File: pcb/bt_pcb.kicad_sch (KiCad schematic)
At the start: 1 part, among them IC4 STM32H750VBT6

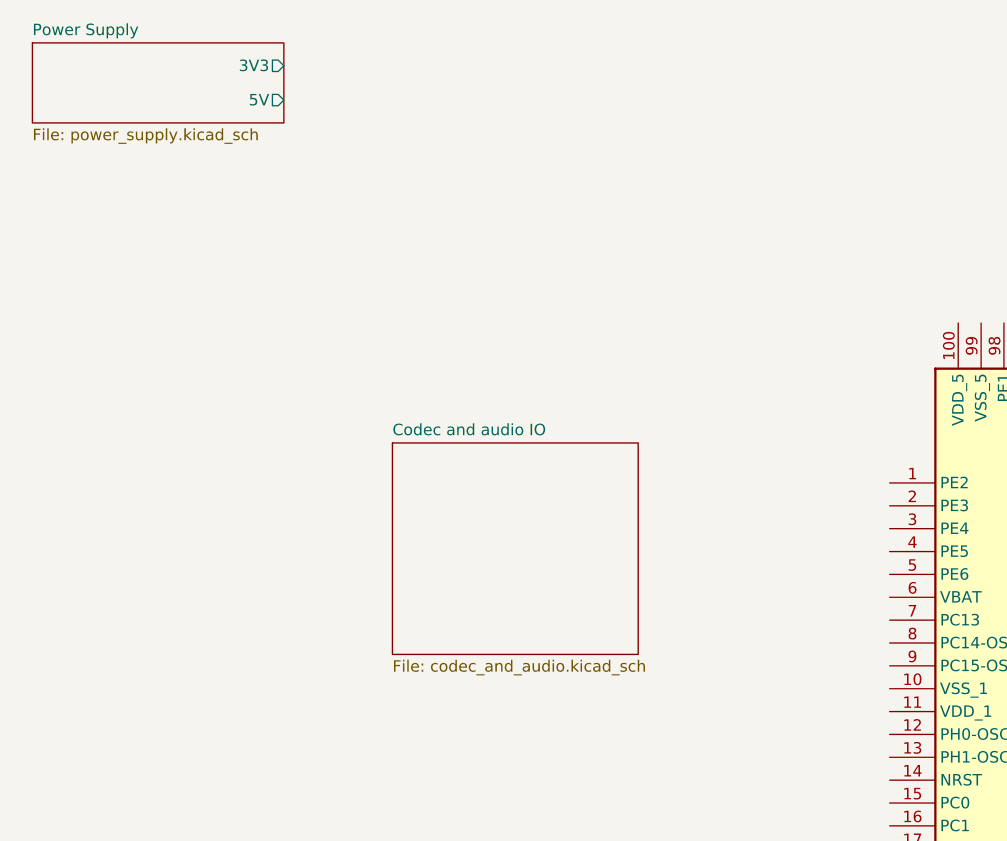
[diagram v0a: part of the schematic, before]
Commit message: progress on audio pcb
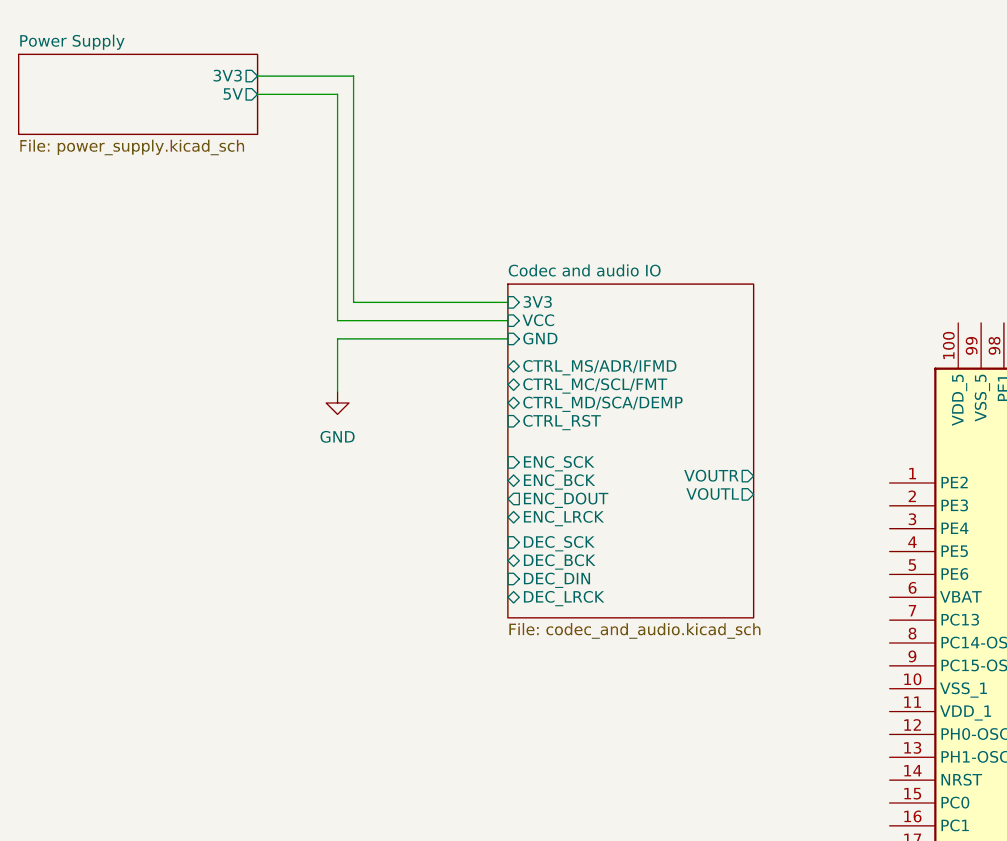
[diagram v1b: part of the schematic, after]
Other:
- sheet Codec and audio IO ports: added 3V3, CTRL_MC/SCL/FMT, CTRL_MD/SCA/DEMP, CTRL_MS/ADR/IFMD, CTRL_RST, DEC_BCK, DEC_DIN, DEC_LRCK, DEC_SCK, ENC_BCK, ENC_DOUT, ENC_LRCK, ENC_SCK, GND, VCC, VOUTL, VOUTR; removed none
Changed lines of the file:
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@@
 (kicad_sch (version 20230121) (generator eeschema)
   (paper "A4")
+  (wire (pts (xy 71.882 67.564) (xy 89.027 67.564))
+    (stroke (width 0) (type default))
+  )
+  (wire (pts (xy 61.214 42.418) (xy 71.882 42.418))
+    (stroke (width 0) (type default))
+  )
+  (wire (pts (xy 71.882 42.418) (xy 71.882 67.564))
+    (stroke (width 0) (type default))
+  )
+  (wire (pts (xy 89.027 69.596) (xy 70.104 69.596))
+    (stroke (width 0) (type default))
+  )
+  (wire (pts (xy 70.104 71.628) (xy 70.104 77.47))
+    (stroke (width 0) (type default))
+  )
+  (wire (pts (xy 70.104 69.596) (xy 70.104 44.45))
+    (stroke (width 0) (type default))
+  )
+  (wire (pts (xy 61.214 44.45) (xy 70.104 44.45))
+    (stroke (width 0) (type default))
+  )
+  (wire (pts (xy 89.027 71.628) (xy 70.104 71.628))
+    (stroke (width 0) (type default))
+  )
+  (symbol (lib_id "power:GND") (at 70.104 77.47 0) (unit 1)
+    (in_bom yes) (on_board yes) (dnp no) (fields_autoplaced)
+    (property "Reference" "#PWR07" (at 70.104 83.82 0)
+      (effects (font (size 1.27 1.27)) hide)
+    )
+    (property "Value" "GND" (at 70.104 82.55 0)
+      (effects (font (size 1.27 1.27)))
+    )
+    (property "Footprint" "" (at 70.104 77.47 0)
+      (effects (font (size 1.27 1.27)) hide)
+    )
+    (property "Datasheet" "" (at 70.104 77.47 0)
+      (effects (font (size 1.27 1.27)) hide)
+    )
+    (pin "1")
+    (instances
+      (project "bt_pcb"
+        (path "/eb787481-08cd-41a4-a128-173fa6227c32"
+          (reference "#PWR07") (unit 1)
+        )
+      )
+    )
+  )
   (symbol (lib_id "SamacSys_Parts:STM32H750VBT6") (at 131.445 87.63 0) (unit 1)
     (in_bom yes) (on_board yes) (dnp no) (fields_autoplaced)
@@
     )
   )
-  (sheet (at 76.2 83.185) (size 27.305 23.495) (fields_autoplaced)
+  (sheet (at 89.027 65.532) (size 27.305 37.084) (fields_autoplaced)
     (stroke (width 0.1524) (type solid))
     (fill (color 0 0 0 0.0000))
-    (property "Sheetname" "Codec and audio IO" (at 76.2 82.4734 0)
+    (property "Sheetname" "Codec and audio IO" (at 89.027 64.8204 0)
       (effects (font (size 1.27 1.27)) (justify left bottom))
     )
-    (property "Sheetfile" "codec_and_audio.kicad_sch" (at 76.2 107.2646 0)
+    (property "Sheetfile" "codec_and_audio.kicad_sch" (at 89.027 103.2006 0)
       (effects (font (size 1.27 1.27)) (justify left top))
+    )
+    (pin "3V3" input (at 89.027 67.564 180)
+      (effects (font (size 1.27 1.27)) (justify left))
+    )
+    (pin "CTRL_MC{slash}SCL{slash}FMT" bidirectional (at 89.027 76.708 180)
+      (effects (font (size 1.27 1.27)) (justify left))
+    )
+    (pin "CTRL_MD{slash}SCA{slash}DEMP" bidirectional (at 89.027 78.74 180)
+      (effects (font (size 1.27 1.27)) (justify left))
+    )
+    (pin "ENC_LRCK" bidirectional (at 89.027 91.44 180)
+      (effects (font (size 1.27 1.27)) (justify left))
+    )
+    (pin "ENC_SCK" input (at 89.027 85.344 180)
+      (effects (font (size 1.27 1.27)) (justify left))
+    )
+    (pin "ENC_DOUT" output (at 89.027 89.408 180)
+      (effects (font (size 1.27 1.27)) (justify left))
+    )
+    (pin "ENC_BCK" bidirectional (at 89.027 87.376 180)
+      (effects (font (size 1.27 1.27)) (justify left))
+    )
+    (pin "GND" input (at 89.027 71.628 180)
+      (effects (font (size 1.27 1.27)) (justify left))
+    )
+    (pin "VCC" input (at 89.027 69.596 180)
+      (effects (font (size 1.27 1.27)) (justify left))
+    )
+    (pin "VOUTR" output (at 116.332 86.868 0)
+      (effects (font (size 1.27 1.27)) (justify right))
+    )
+    (pin "VOUTL" output (at 116.332 88.9 0)
+      (effects (font (size 1.27 1.27)) (justify right))
+    )
+    (pin "CTRL_RST" input (at 89.027 80.772 180)
+      (effects (font (size 1.27 1.27)) (justify left))
+    )
+    (pin "DEC_DIN" input (at 89.027 98.298 180)
+      (effects (font (size 1.27 1.27)) (justify left))
+    )
+    (pin "CTRL_MS{slash}ADR{slash}IFMD" bidirectional (at 89.027 74.676 180)
+      (effects (font (size 1.27 1.27)) (justify left))
+    )
+    (pin "DEC_LRCK" bidirectional (at 89.027 100.33 180)
+      (effects (font (size 1.27 1.27)) (justify left))
+    )
+    (pin "DEC_SCK" input (at 89.027 94.234 180)
+      (effects (font (size 1.27 1.27)) (justify left))
+    )
+    (pin "DEC_BCK" bidirectional (at 89.027 96.266 180)
+      (effects (font (size 1.27 1.27)) (justify left))
     )
     (instances
@@
     )
   )
-  (sheet (at 36.195 38.735) (size 27.94 8.89) (fields_autoplaced)
+  (sheet (at 34.671 40.005) (size 26.543 8.89) (fields_autoplaced)
     (stroke (width 0.1524) (type solid))
     (fill (color 0 0 0 0.0000))
-    (property "Sheetname" "Power Supply" (at 36.195 38.0234 0)
+    (property "Sheetname" "Power Supply" (at 34.671 39.2934 0)
       (effects (font (size 1.27 1.27)) (justify left bottom))
     )
-    (property "Sheetfile" "power_supply.kicad_sch" (at 36.195 48.2096 0)
+    (property "Sheetfile" "power_supply.kicad_sch" (at 34.671 49.4796 0)
       (effects (font (size 1.27 1.27)) (justify left top))
     )
-    (pin "3V3" output (at 64.135 41.275 0)
-      (effects (font (size 1.27 1.27)) (justify right))
-    )
-    (pin "5V" output (at 64.135 45.085 0)
-      (effects (font (size 1.27 1.27)) (justify right))
-    )
+    (pin "3V3" output (at 61.214 42.418 0)
+      (effects (font (size 1.27 1.27)) (justify right))
+    )
+    (pin "5V" output (at 61.214 44.45 0)
+      (effects (font (size 1.27 1.27)) (justify right))
+    )

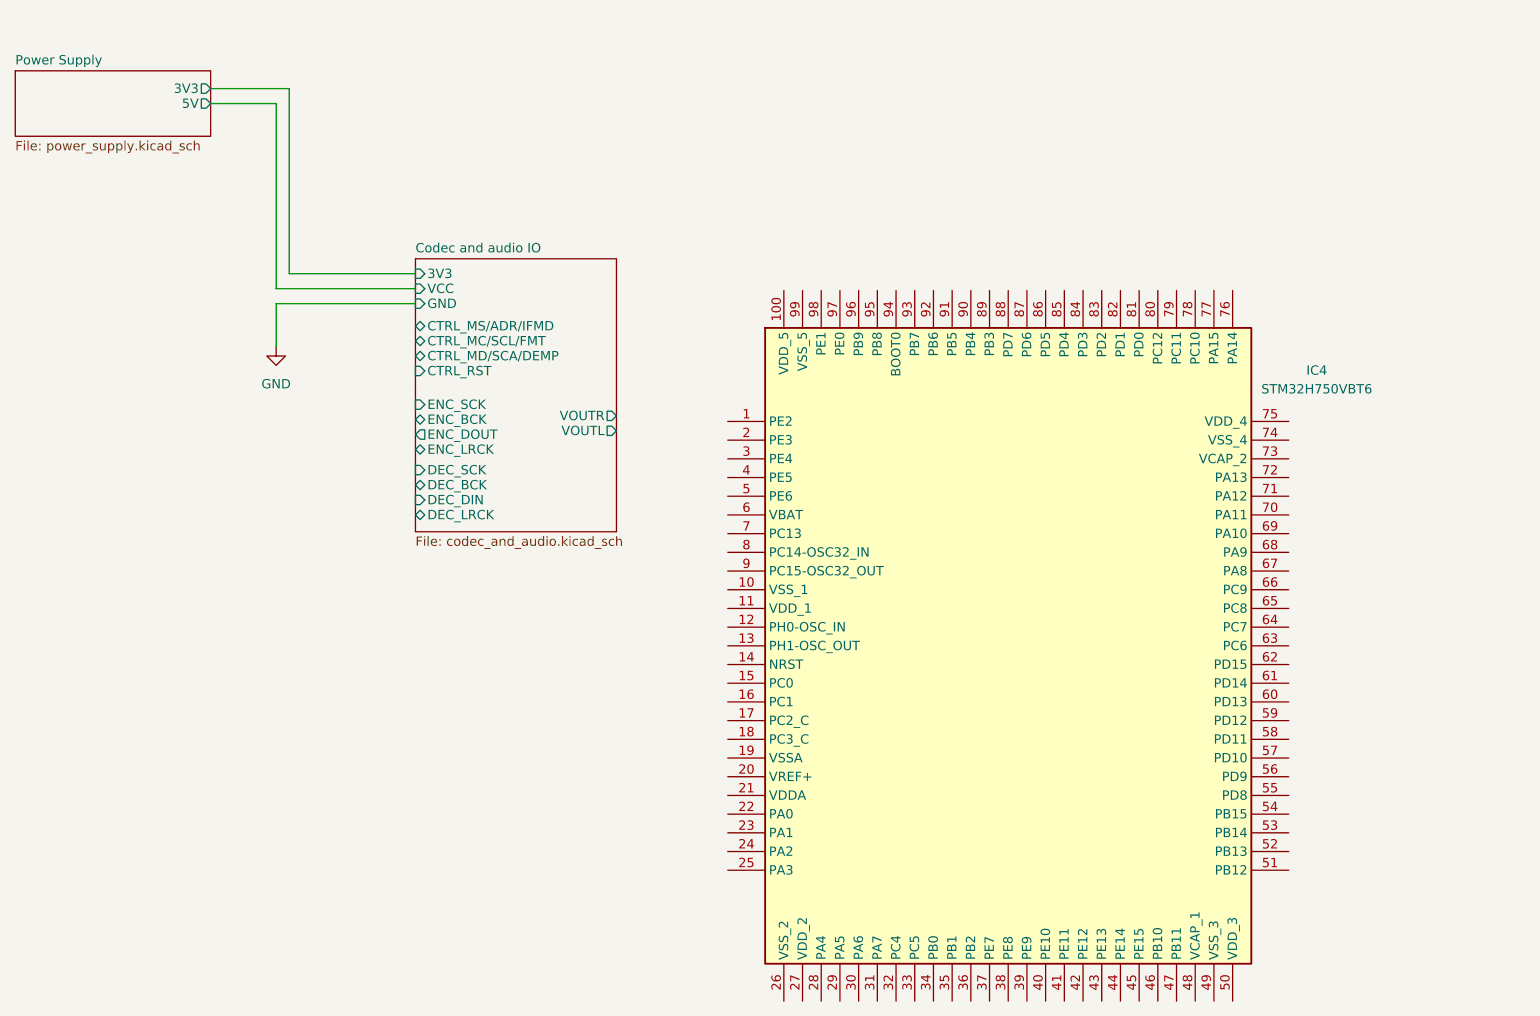
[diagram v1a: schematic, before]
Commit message: progress on understanding audio schematics
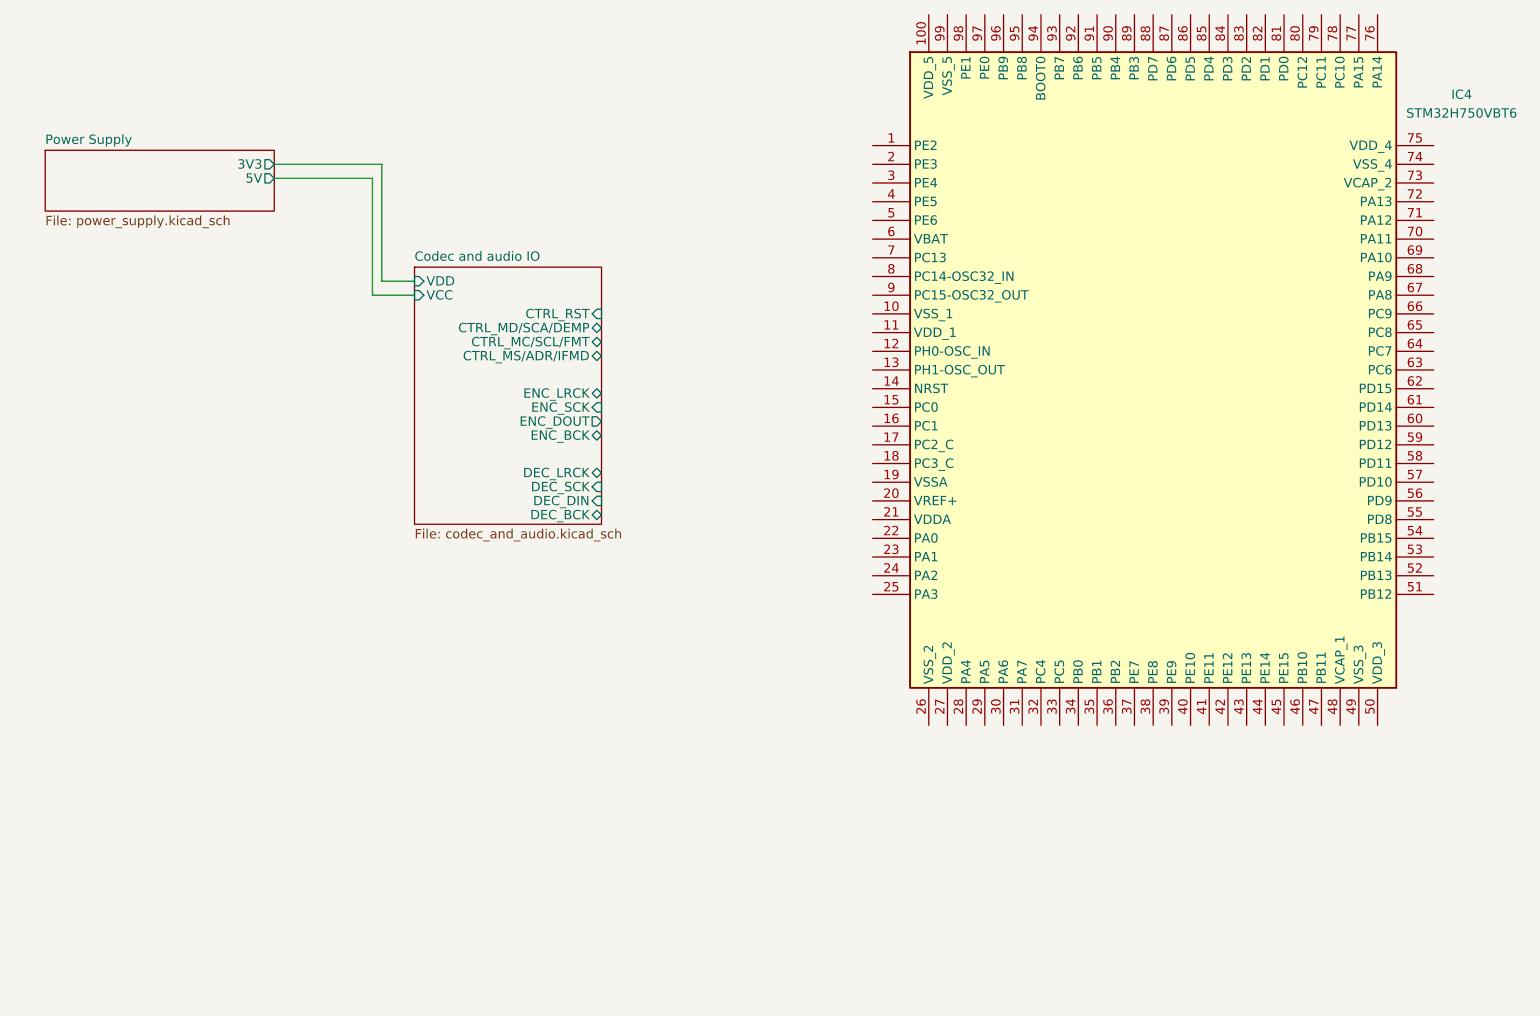
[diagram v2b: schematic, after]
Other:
- sheet Codec and audio IO ports: added VDD; removed 3V3, GND, VOUTL, VOUTR
- moved on the sheet: IC4
